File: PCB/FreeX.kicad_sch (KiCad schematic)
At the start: 12 parts, among them J1 2-1734839-4, J2 TF31-6S-0.5SH_800_, J3 USB4105-GF-A, J4 54-00177, U1 W25Q32JVZPIQ, U2 MPU-9250, U3 ESP32-D0WDQ6, U4 CP2102, U5 TC2014-3.3VxCTTR, U6 LM358PW, U7 TDA7052AT_N2, Y1 WE-SPXO_IQXO-791

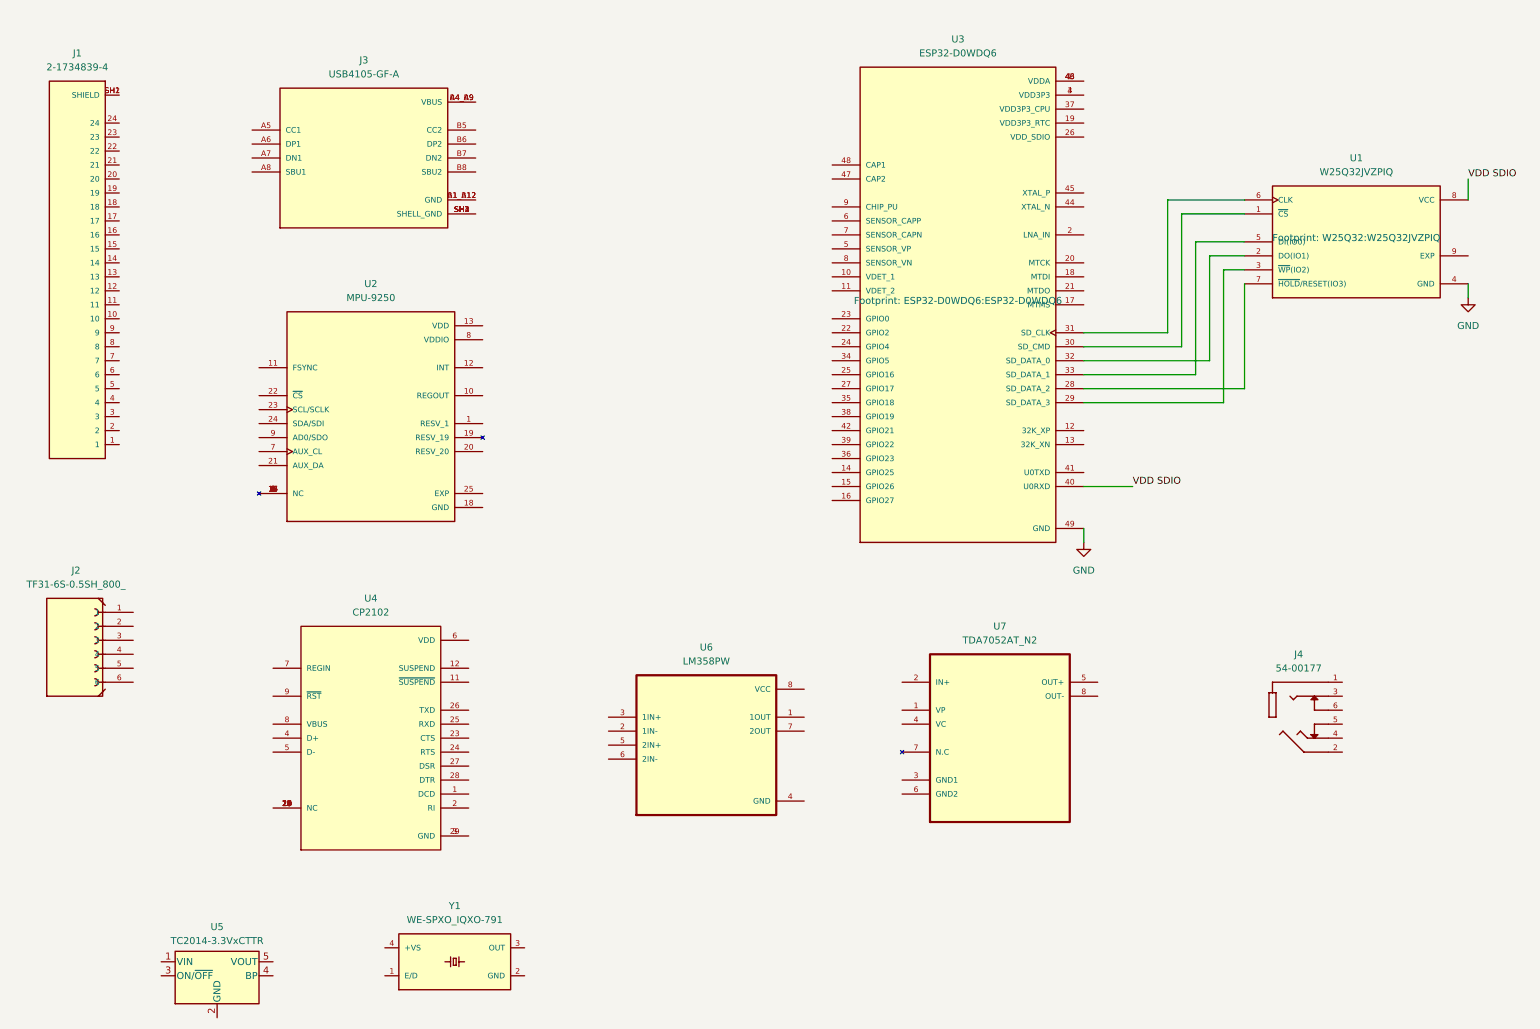
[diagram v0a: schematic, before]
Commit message: 14th, march. 2025
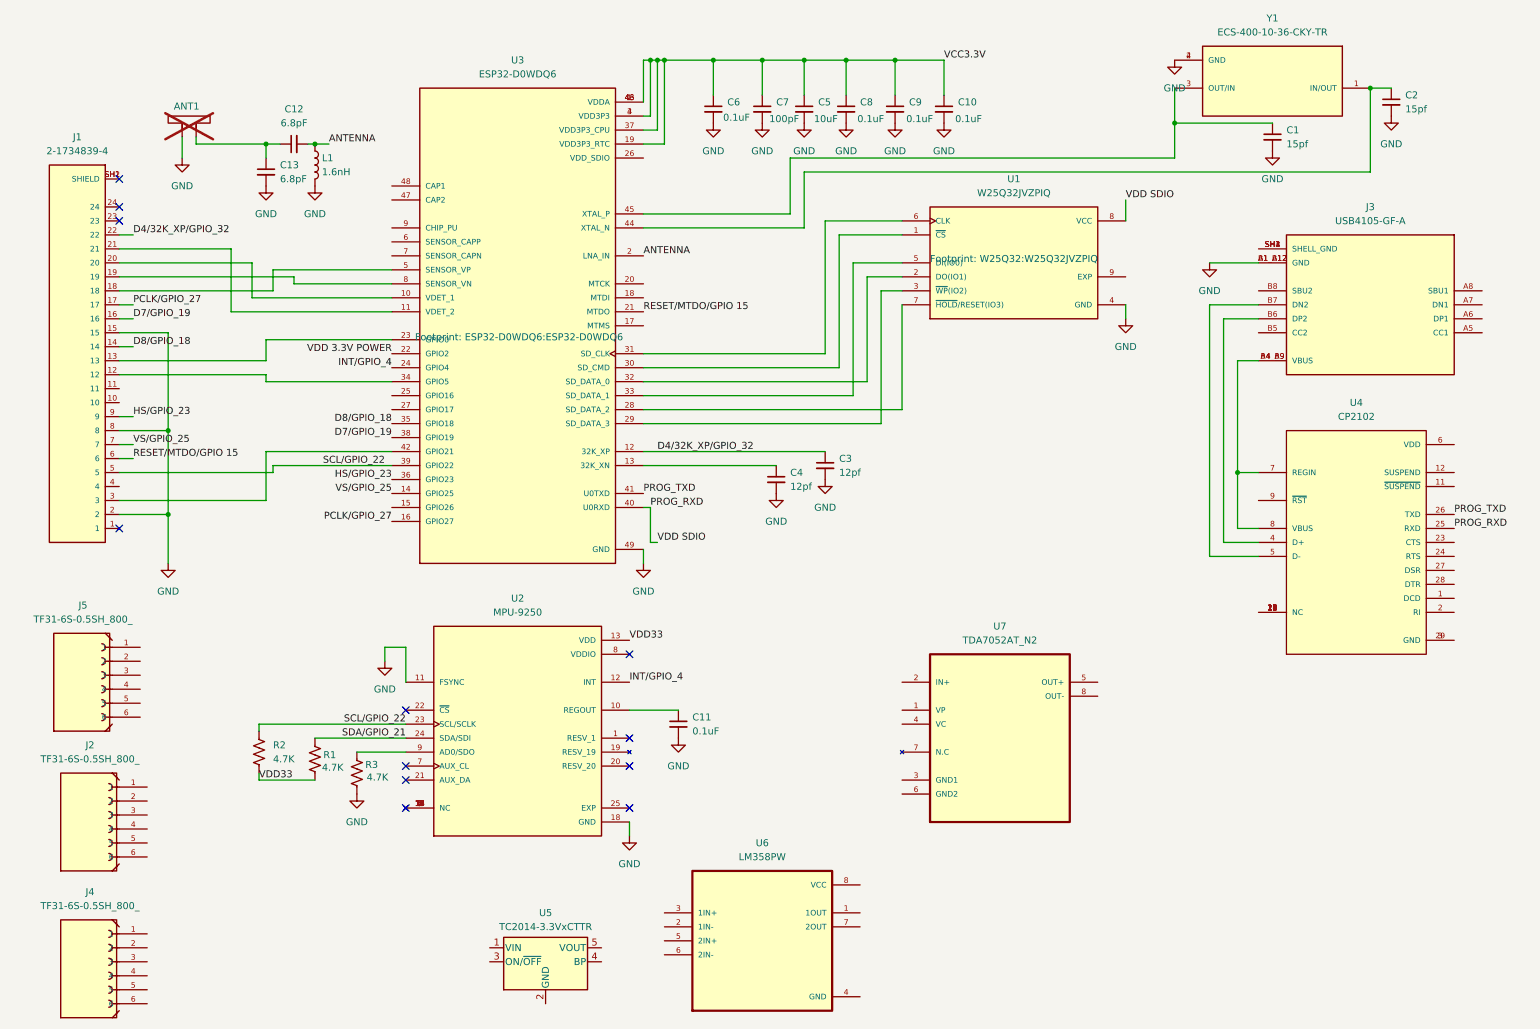
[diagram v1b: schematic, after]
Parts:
- removed J4: 54-00177, 54-00177-Headphone-Jack:54-00177-Headphone-Jack, symbol 54-00177-Headphone-Jack:54-00177
- removed Y1: WE-SPXO_IQXO-791, STP_831056298-Crystal-Oscillator:STP_831056298-Crystal-Oscillator, symbol STP_831056298-Crystal-Oscillator:WE-SPXO_IQXO-791
- added ANT1: Antenna_Dipole, symbol Device:Antenna_Dipole
- added C1, C2: 15pf, Capacitor_SMD:C_0201_0603Metric, symbol Device:C_Small
- added C10, C11, C6, C8, C9: 0.1uF, Capacitor_SMD:C_0201_0603Metric, symbol Device:C_Small
- added C12, C13: 6.8pF, Capacitor_SMD:C_0201_0603Metric, symbol Device:C_Small
- added C3, C4: 12pf, Capacitor_SMD:C_0201_0603Metric, symbol Device:C_Small
- added C5: 10uF, Capacitor_SMD:C_0201_0603Metric, symbol Device:C_Small
- added C7: 100pF, Capacitor_SMD:C_0201_0603Metric, symbol Device:C_Small
- added J4, J5: TF31-6S-0.5SH_800_, TF31-6S-0.5SH_800-6-pins:TF31-6S-0.5SH_800-6-pins, symbol TF31-6S-0.5SH_800-6-pins:TF31-6S-0.5SH_800_
- added L1: 1.6nH, Inductor_SMD:L_0201_0603Metric, symbol Device:L
- added R1, R2, R3: 4.7K, Resistor_SMD:R_0201_0603Metric, symbol Device:R_US
- added Y1: ECS-400-10-36-CKY-TR, 40 MHz_±10ppm_Crystal_10pF_40_Ohms_4-SMD:ECS-400-10-36-CKY-TR, symbol 40 MHz_±10ppm_Crystal_10pF_40_Ohms_4-SMD:ECS-400-10-36-CKY-TR
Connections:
- net VDD SDIO is gone; now on net PROG_RXD: U1.8 (VCC), U3.40 (U0RXD)
- net GND: now also J1.15, J1.2, J1.8, J3.A1_B12 (GND), J3.B1_A12 (GND), U2.11 (FSYNC), U2.18 (GND), ANT1.1, C1.2, C10.2, C11.2, C13.2, C2.2, C3.2, C4.2, C5.2, C6.2, C7.2, C8.2, C9.2, L1.2, R3.2, Y1.2 (GND), Y1.4 (GND)
- net VCC3.3V: now reaches U3.1 (VDDA), U3.43 (VDDA), U3.46 (VDDA)
- net VCC3.3V: now also U3.19 (VDD3P3_RTC), U3.3 (VDD3P3), U3.37 (VDD3P3_CPU), U3.4 (VDD3P3), C10.1, C5.1, C6.1, C7.1, C8.1, C9.1
- net at U3.10 (VDET_1): now also J1.20
- net at U3.11 (VDET_2): now also J1.21
- net D4/32K_XP/GPIO_32: now reaches U3.12 (32K_XP)
- net D4/32K_XP/GPIO_32: now also J1.22, C3.1
- net at U3.13 (32K_XN): now also C4.1
- net VS/GPIO_25: now reaches U3.14 (GPIO25)
- net VS/GPIO_25: now also J1.7
- net PCLK/GPIO_27: now reaches U3.16 (GPIO27)
- net PCLK/GPIO_27: now also J1.17
- net ANTENNA: now reaches U3.2 (LNA_IN)
- net ANTENNA: now also C12.2, L1.1
- net RESET/MTDO/GPIO 15: now reaches U3.21 (MTDO)
- net RESET/MTDO/GPIO 15: now also J1.6
- net VDD 3.3V POWER: now reaches U3.22 (GPIO2)
- net at U3.23 (GPIO0): now also J1.13
- net INT/GPIO_4: now reaches U3.24 (GPIO4)
- net INT/GPIO_4: now also U2.12 (INT)
- net at U3.34 (GPIO5): now also J1.12
- net D8/GPIO_18: now reaches U3.35 (GPIO18)
- net D8/GPIO_18: now also J1.14
- net HS/GPIO_23: now reaches U3.36 (GPIO23)
- net HS/GPIO_23: now also J1.9
- net D7/GPIO_19: now reaches U3.38 (GPIO19)
- net D7/GPIO_19: now also J1.16
- net SCL/GPIO_22: now reaches U3.39 (GPIO22)
- net SCL/GPIO_22: now also J1.5, U2.23 (SCL/SCLK), R2.1
- net PROG_TXD: now reaches U3.41 (U0TXD)
- net PROG_TXD: now also U4.26 (TXD)
- net at U3.42 (GPIO21): now also J1.3
- net at U3.44 (XTAL_N): now also C2.1, Y1.1 (IN/OUT)
- net at U3.45 (XTAL_P): now also C1.1, Y1.3 (OUT/IN)
- net at U3.5 (SENSOR_VP): now also J1.18
- net at U3.8 (SENSOR_VN): now also J1.19
- net at U2.10 (REGOUT): now also C11.1
- net VDD33: now reaches U2.13 (VDD)
- net VDD33: now also R1.2, R2.2
- net SDA/GPIO_21: now reaches U2.24 (SDA/SDI)
- net SDA/GPIO_21: now also R1.1
- net at U2.9 (AD0/SDO): now also R3.1
- net at J3.A4_B9 (VBUS), J3.B4_A9 (VBUS): now also U4.7 (REGIN), U4.8 (VBUS)
- net at J3.B6 (DP2): now also U4.4 (D+)
- net at J3.B7 (DN2): now also U4.5 (D-)
- net PROG_RXD: now reaches U4.25 (RXD)
- new net: ANT1.2, C12.1, C13.1
- no-connect marks 0 -> 12
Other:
- moved on the sheet: J1, J2, J3, U1, U2, U3, U4, U5, U6
